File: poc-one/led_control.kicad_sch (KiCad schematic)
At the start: 49 parts, among them Q1 SS8550 Y2 200-350, Q2 SS8550 Y2 200-350, Q3 SS8550 Y2 200-350, Q5 SS8550 Y2 200-350, U10 74HC595D, U11 74HC595D, U12 74HC595D, U13 74HC595D, U14 74HC595D, U15 74HC595D, U16 74HC595D, U17 74HC595D, U18 74HC595D, U19 74HC595D, U20 74HC595D, U4 74HC138, U5 74HC138, U6 74HC138, U7 74HC138, U8 74HC138, U9 74HC595D

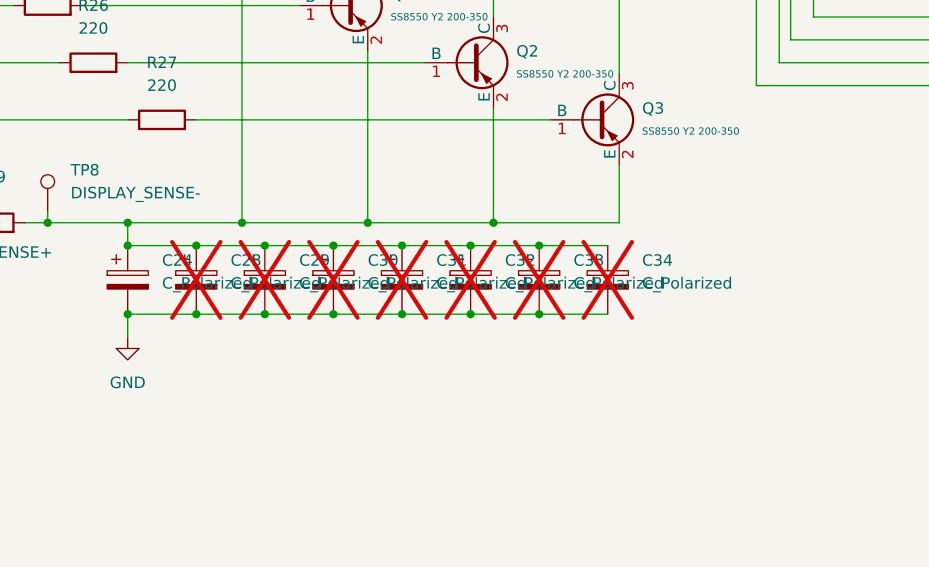
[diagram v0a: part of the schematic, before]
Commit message: poc-one update & bom
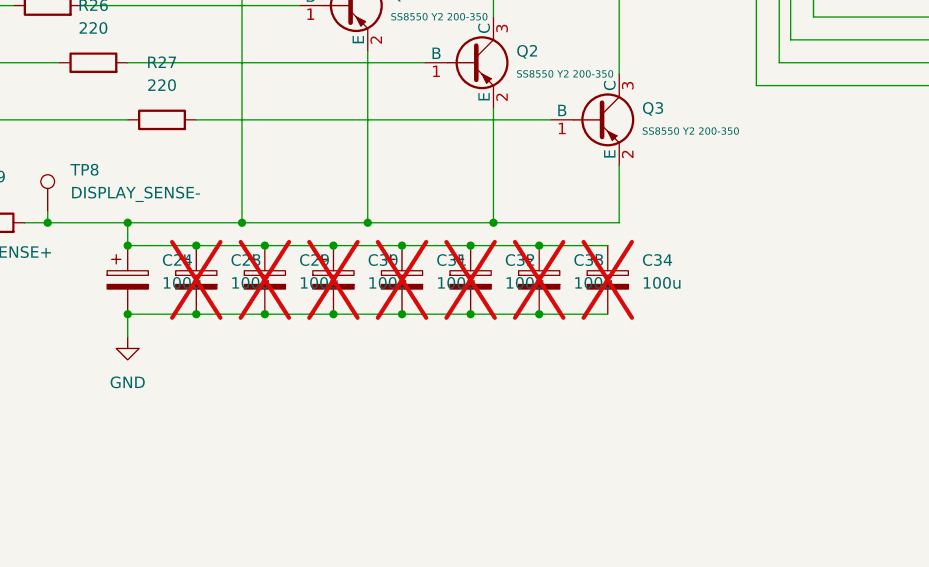
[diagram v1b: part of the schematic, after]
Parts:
- C24, C28, C29, C30, C31, C32, C33, C34: value C_Polarized -> 100u
- R39: footprint (none) -> Resistor_SMD:R_0402_1005Metric
- TP8, TP9: footprint (none) -> TestPoint:TestPoint_Pad_D1.5mm
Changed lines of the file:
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@@
 	)
 	(junction
-		(at 175.26 171.45)
+		(at 213.36 179.07)
 		(diameter 0)
 		(color 0 0 0 0)
 	)
 	(junction
-		(at 213.36 179.07)
+		(at 205.74 179.07)
 		(diameter 0)
 		(color 0 0 0 0)
 	)
 	(junction
-		(at 205.74 179.07)
+		(at 175.26 179.07)
 		(diameter 0)
 		(color 0 0 0 0)
@@
 	)
 	(junction
-		(at 175.26 179.07)
-		(diameter 0)
-		(color 0 0 0 0)
-	)
-	(junction
 		(at 190.5 179.07)
 		(diameter 0)
@@
 	)
 	(junction
+		(at 175.26 171.45)
+		(diameter 0)
+		(color 0 0 0 0)
+	)
+	(junction
 		(at 355.6 87.63)
 		(diameter 0)
@@
 		(exclude_from_sim no)
 		(in_bom yes)
-		(on_board yes)
+		(on_board no)
 		(in_pos_files yes)
 		(dnp yes)
@@
 			)
 		)
-		(property "Value" "C_Polarized"
+		(property "Value" "100u"
 			(at 186.69 175.6409 0)
 			(show_name no)
@@
 		(exclude_from_sim no)
 		(in_bom yes)
-		(on_board yes)
+		(on_board no)
 		(in_pos_files yes)
 		(dnp yes)
@@
 			)
 		)
-		(property "Value" "C_Polarized"
+		(property "Value" "100u"
 			(at 201.93 175.6409 0)
 			(show_name no)
@@
 		(exclude_from_sim no)
 		(in_bom yes)
-		(on_board yes)
+		(on_board no)
 		(in_pos_files yes)
 		(dnp yes)
@@
 			)
 		)
-		(property "Value" "C_Polarized"
+		(property "Value" "100u"
 			(at 217.17 175.6409 0)
 			(show_name no)
@@
 		(exclude_from_sim no)
 		(in_bom yes)
-		(on_board yes)
+		(on_board no)
 		(in_pos_files yes)
 		(dnp yes)
@@
 			)
 		)
-		(property "Value" "C_Polarized"
+		(property "Value" "100u"
 			(at 224.79 175.6409 0)
 			(show_name no)
@@
 			)
 		)
-		(property "Value" "C_Polarized"
+		(property "Value" "100u"
 			(at 179.07 175.6409 0)
 			(show_name no)
@@
 		(exclude_from_sim no)
 		(in_bom yes)
-		(on_board yes)
+		(on_board no)
 		(in_pos_files yes)
 		(dnp yes)
@@
 			)
 		)
-		(property "Value" "C_Polarized"
+		(property "Value" "100u"
 			(at 194.31 175.6409 0)
 			(show_name no)
@@
 		(exclude_from_sim no)
 		(in_bom yes)
-		(on_board yes)
+		(on_board no)
 		(in_pos_files yes)
 		(dnp yes)
@@
 			)
 		)
-		(property "Value" "C_Polarized"
+		(property "Value" "100u"
 			(at 209.55 175.6409 0)
 			(show_name no)
@@
 			)
 		)
-		(property "Footprint" ""
+		(property "Footprint" "TestPoint:TestPoint_Pad_D1.5mm"
 			(at 171.45 167.64 0)
 			(hide yes)
@@
 			)
 		)
-		(property "Footprint" ""
+		(property "Footprint" "Resistor_SMD:R_0402_1005Metric"
 			(at 160.02 170.688 90)
 			(hide yes)
@@
 		(exclude_from_sim no)
 		(in_bom yes)
-		(on_board yes)
+		(on_board no)
 		(in_pos_files yes)
 		(dnp yes)
@@
 			)
 		)
-		(property "Value" "C_Polarized"
+		(property "Value" "100u"
 			(at 232.41 175.6409 0)
 			(show_name no)
@@
 			)
 		)
-		(property "Footprint" ""
+		(property "Footprint" "TestPoint:TestPoint_Pad_D1.5mm"
 			(at 157.48 168.91 0)
 			(hide yes)
